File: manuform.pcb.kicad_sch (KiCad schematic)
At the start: 11 parts, among them J1 Conn_01x05, J3 Conn_01x01, J4 Conn_01x01, SW1 SW_DIP_x01, SW2 SW_DIP_x01, SW3 SW_DIP_x01, SW4 SW_DIP_x01

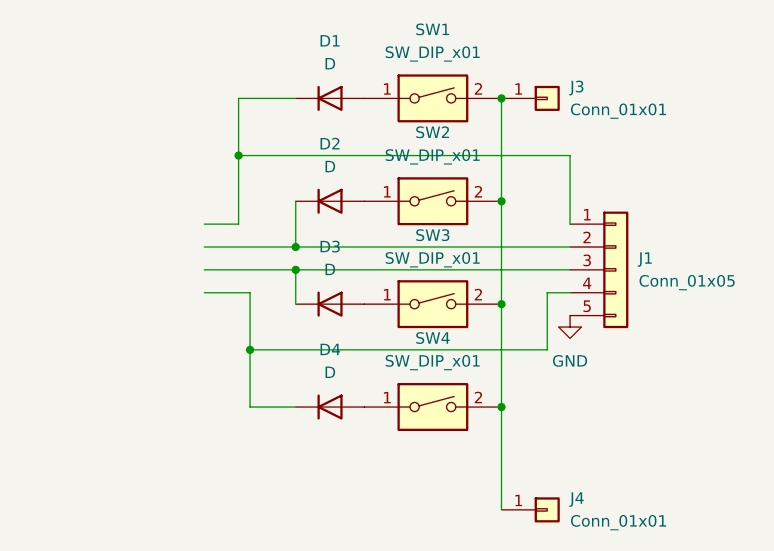
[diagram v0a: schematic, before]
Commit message: kalih choc v2 flex PCB
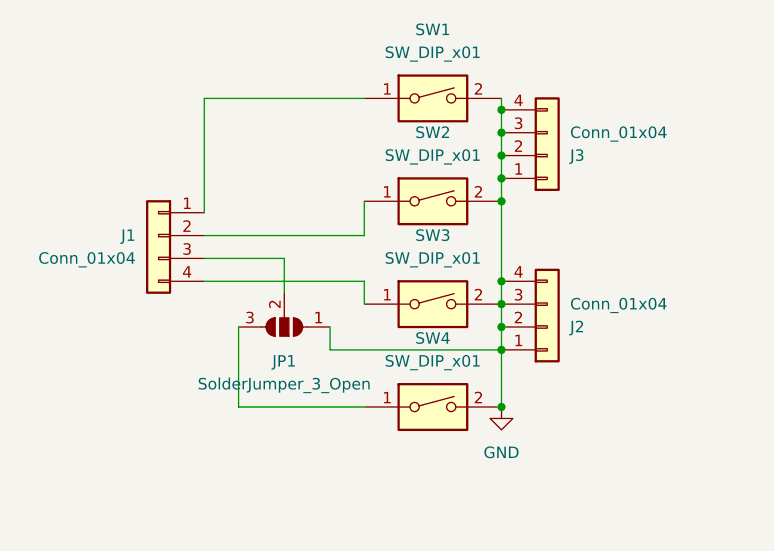
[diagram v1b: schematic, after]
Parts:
- removed D1, D2, D3, D4: D, Diode_SMD:D_SOD-123, symbol Device:D
- removed J3, J4: Conn_01x01, Connector_PinHeader_2.54mm:PinHeader_1x01_P2.54mm_Vertical, symbol Connector_Generic:Conn_01x01
- added J2, J3: Conn_01x04, Connector_PinHeader_2.00mm:PinHeader_1x04_P2.00mm_Vertical, symbol Connector_Generic:Conn_01x04
- added JP1: SolderJumper_3_Open, Jumper:SolderJumper-3_P2.0mm_Open_TrianglePad1.0x1.5mm_NumberLabels, symbol Jumper:SolderJumper_3_Open
- J1: value Conn_01x05 -> Conn_01x04; footprint Connector_PinHeader_2.54mm:PinHeader_1x05_P2.54mm_Vertical -> Connector_PinHeader_2.00mm:PinHeader_1x04_P2.00mm_Horizontal; symbol Connector_Generic:Conn_01x05 -> Connector_Generic:Conn_01x04
- SW1, SW2, SW3, SW4: footprint switchCustom:SW_Cherry_MX_1.00u_PCB -> switchCustom:SW_Kailh_Choc_V2_elongated
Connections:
- net GND: now also SW1.2, SW2.2, SW3.2, SW4.2, J2.1 (Pin_1), J2.2 (Pin_2), J2.3 (Pin_3), J2.4 (Pin_4), J3.1 (Pin_1), J3.2 (Pin_2), J3.3 (Pin_3), J3.4 (Pin_4), JP1.1 (A); no longer J1.5 (Pin_5)
- net at SW2.1: now also J1.2 (Pin_2)
- net at SW3.1: now also J1.4 (Pin_4)
- net at SW1.1: now also J1.1 (Pin_1)
- net at SW4.1: now also JP1.3 (B)
- net at J1.3 (Pin_3): now also JP1.2 (C)
